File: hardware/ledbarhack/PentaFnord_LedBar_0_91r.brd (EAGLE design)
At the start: 100 x 65.3 mm, 113 parts, among them IC1 MEGA8-AI, IC2 MAX487, IC3 78L05, Q1 BSS138, Q2 BSS138, Q3 BSS138, Q4 BSS138, Q5 BSS138, SW1 MCMT5-F-VADAPTED_FOOTPRINT, U1 NICHIA_NSSL157T-H3, U2 NICHIA_NSSL157T-H3, U3 NICHIA_NSSL157T-H3, U4 NICHIA_NSSL157T-H3, U5 NICHIA_NSSL157T-H3, X1 20 MHz

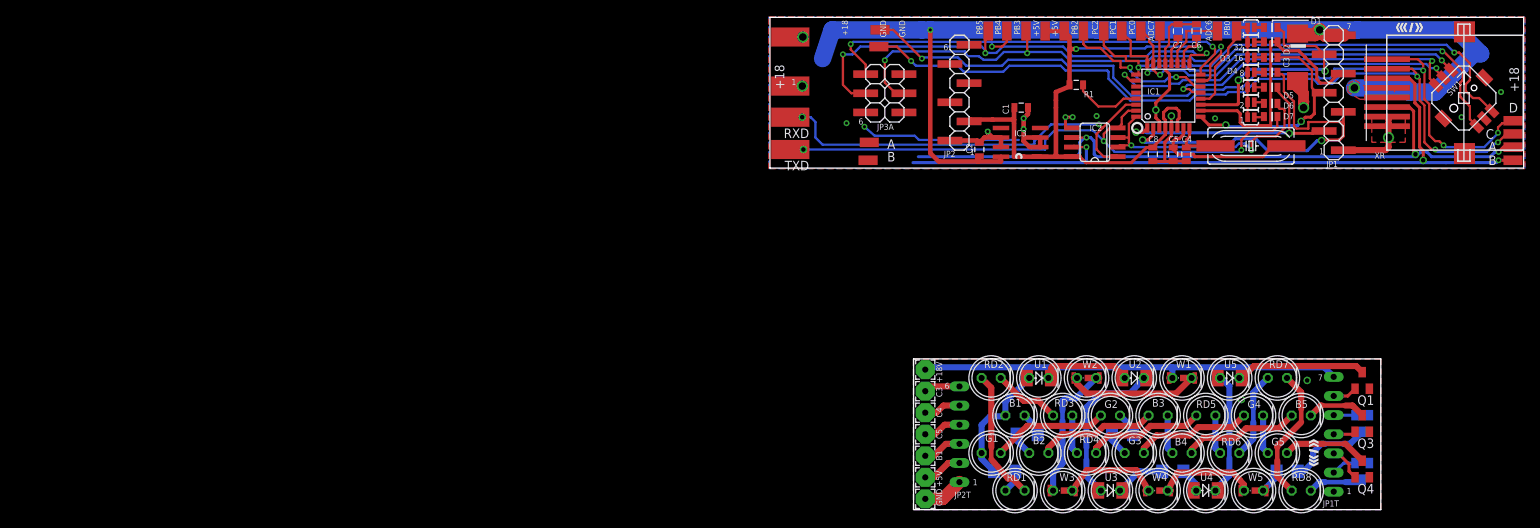
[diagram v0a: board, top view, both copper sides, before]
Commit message: routing done
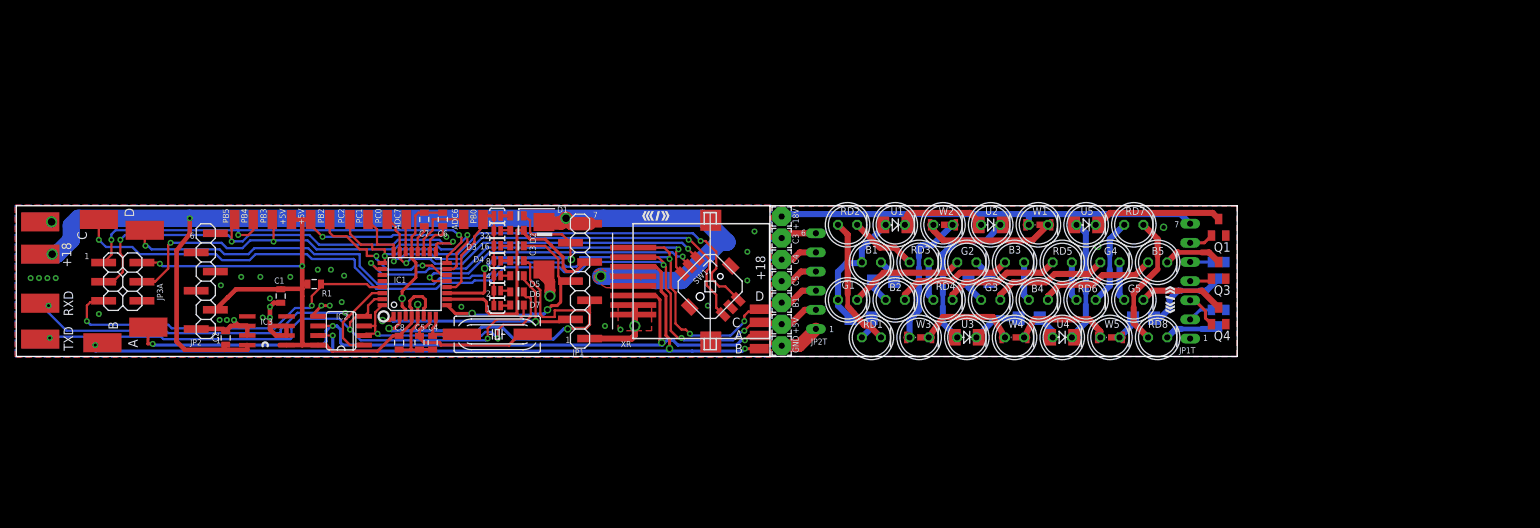
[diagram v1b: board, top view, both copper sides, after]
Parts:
- A_L, B_L: device wirepad:SMD1,27-2,54 -> wirepad:SMD2,54-5,08
- C_L, D_L: value WIREPADSMD1,27-254 -> WIREPADSMD2,54-5,08; device wirepad:SMD1,27-2,54 -> wirepad:SMD2,54-5,08
- moved C_L 106.0 mm to (-89.0, 18.2)
- moved R1 104.5 mm to (-60.5, 9.61)
- moved B_L 104.4 mm to (-88.6, 1.83)
- moved JP3A 104.2 mm to (-84.6, 11.2)
- moved ADC6 103.1 mm to (-40.6, 18.2)
- moved ADC7 103.1 mm to (-48.2, 18.2)
- moved A_R 103.1 mm to (-1.42, 2.78)
- moved B_R 103.1 mm to (-1.42, 1.04)
- moved C 103.1 mm to (-1.42, 4.53)
- moved C2 103.1 mm to (-72.2, 2.46)
- moved C3 103.1 mm to (-30.0, 14.7)
- moved C4 103.1 mm to (-46.5, 1.83)
- moved C5 103.1 mm to (-44.8, 1.83)
- moved C6 103.1 mm to (-43.4, 18.2)
- moved C7 103.1 mm to (-45.9, 18.2)
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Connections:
- net SPARE_B1: now also IC1.13
- net VCC: now also JP3A.2
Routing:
- net VCC: track 87.0 -> 106.2 mm, vias 2 -> 4
- net RST: track 30.3 -> 47.7 mm, vias 1 -> 2
- net RS485B: track 99.1 -> 109.3 mm, vias 3 -> 4
- net N$1: track 105.6 -> 111.5 mm
- net RS485A: track 95.9 -> 100.4 mm, vias 3 -> 4
- net +18V: track 152.3 -> 155.4 mm
- net MOSI: track 63.8 -> 61.0 mm
- net SCK: track 64.8 -> 62.1 mm
- net MISO: track 62.4 -> 59.9 mm
- net N$2: track 108.6 -> 106.3 mm
- net RXD: track 58.7 -> 57.6 mm
- net GND: track 70.5 -> 71.1 mm, vias 15 -> 34
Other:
- board size 100 x 65.3 mm -> 162 x 20 mm
- board text added: "C"
- board text added: "CtrlBoard 0.91r"
- board text added: "D"
- board text removed: "CtrlBoard 0.91"
